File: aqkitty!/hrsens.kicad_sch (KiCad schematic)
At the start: 11 parts, among them U1 ENS160-BGLM, U2 XIAO-RP2040-DIP, U3 OLED_0.91_128x32, U4 SHT30-DIS

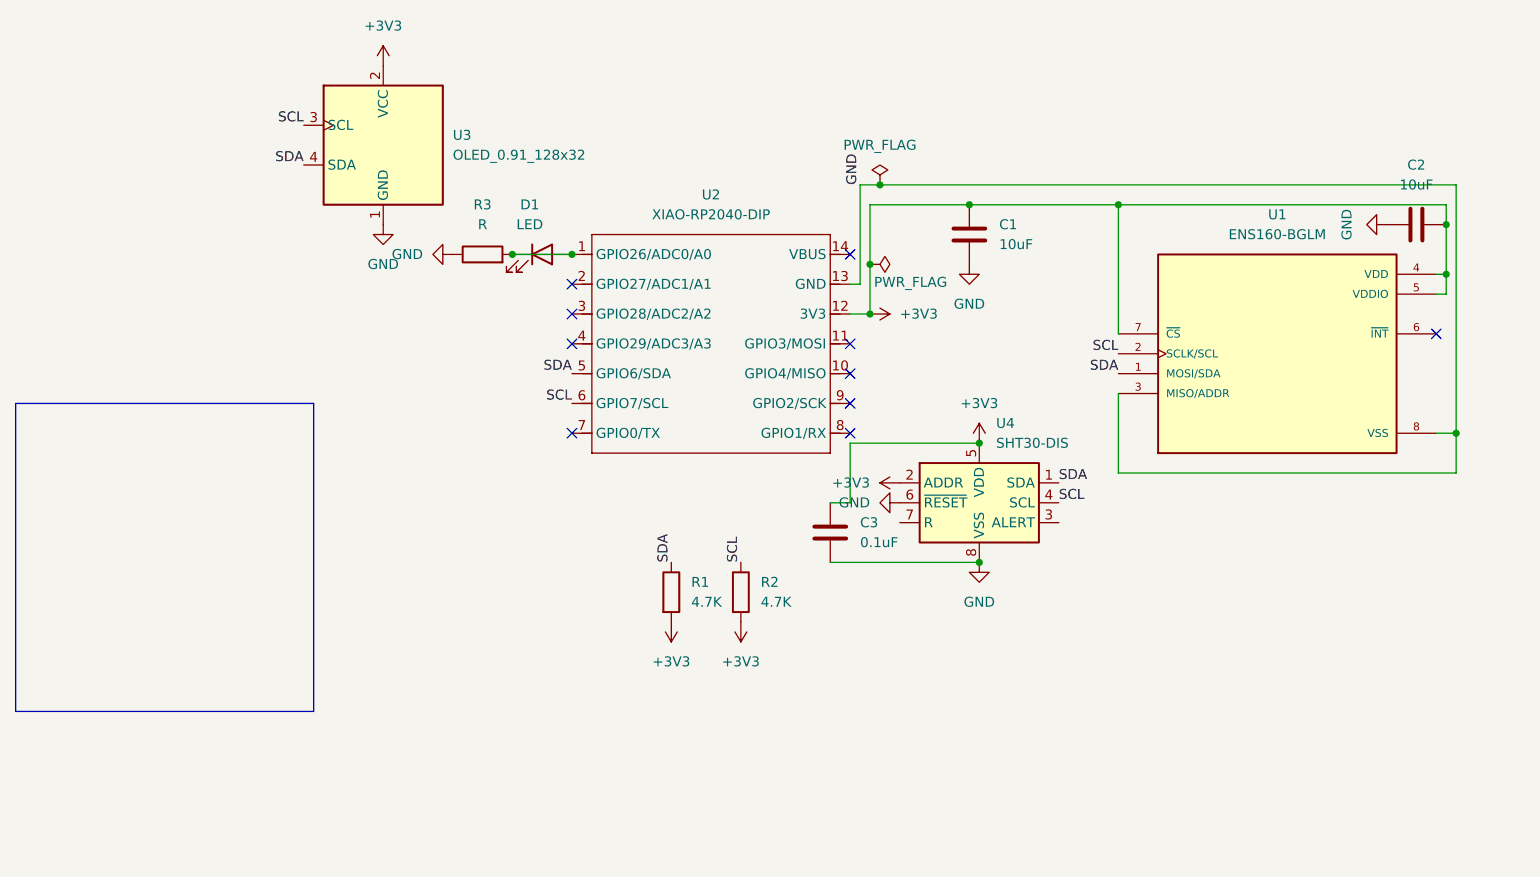
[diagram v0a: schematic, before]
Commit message: yay finished pcb layout
for REAL this time after adding temp sens and also um yes gonna do readme now
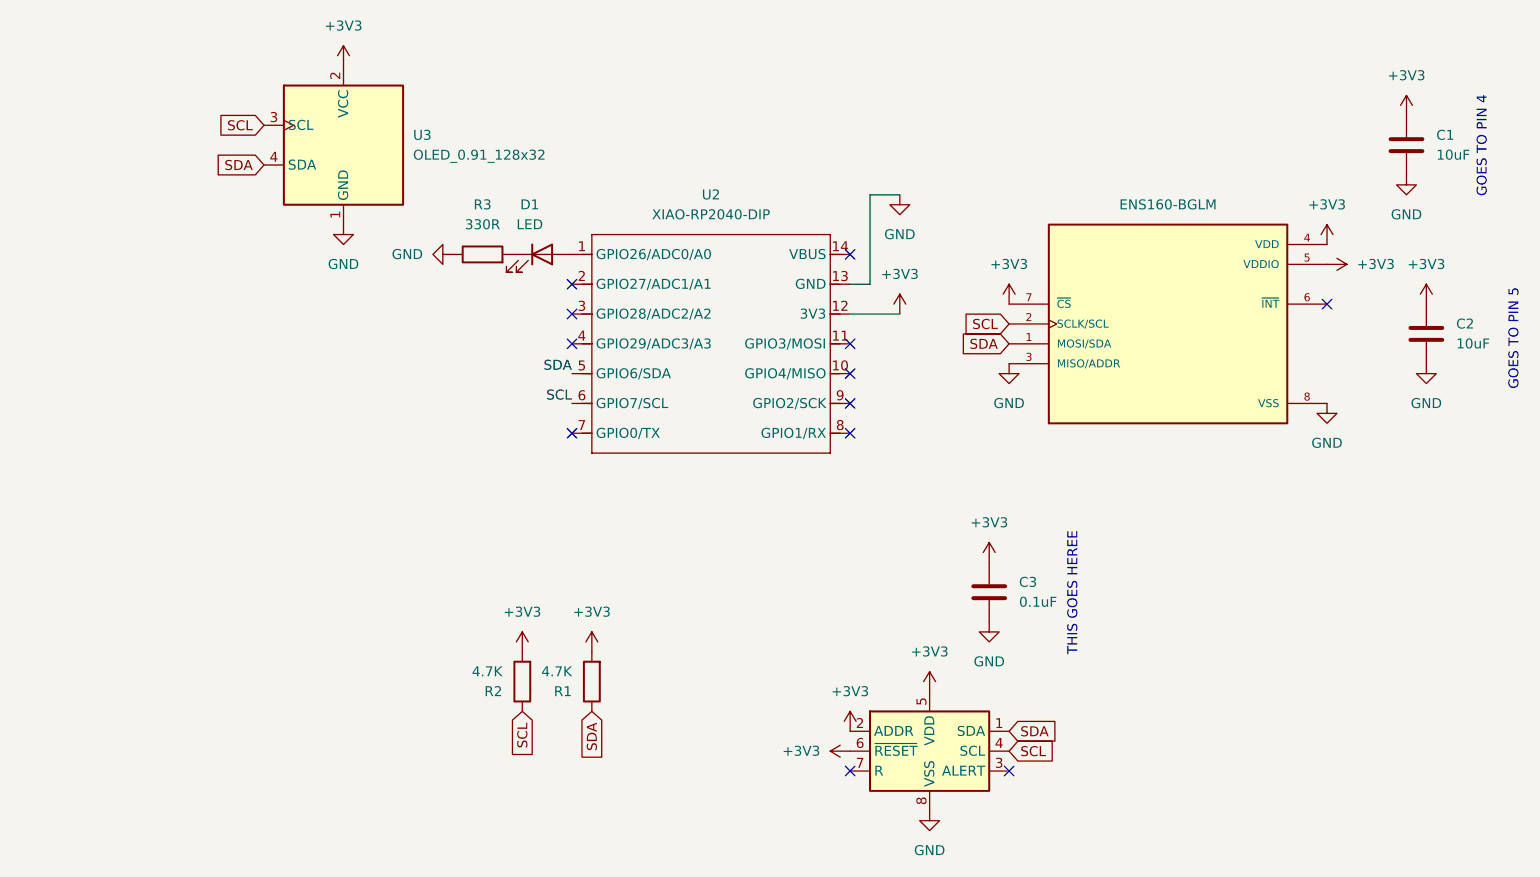
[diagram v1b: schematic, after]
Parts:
- R3: value R -> 330R
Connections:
- net +3V3: now also U4.6 (~{RESET})
- net GND: no longer U4.6 (~{RESET})
- net at D1.1 (K), R3.2: no longer D1.2 (A), U2.1 (GPIO26/ADC0/A0)
- new net: D1.2 (A), U2.1 (GPIO26/ADC0/A0)
- no-connect marks 10 -> 12
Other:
- note added: "GOES TO PIN 4"
- note added: "GOES TO PIN 5"
- note added: "THIS GOES HEREE"
- moved on the sheet: R1, R2, U3
